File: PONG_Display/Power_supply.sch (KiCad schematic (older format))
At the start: 21 parts, among them J2 Input_Supply+12V, U2 MCP16311MS, U3 LD1117S33TR_SOT223

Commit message: v2
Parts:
- C10, C6, C7: footprint Capacitor_THT:CP_Axial_L10.0mm_D4.5mm_P15.00mm_Horizontal -> Capacitor_THT:CP_Radial_D6.3mm_P2.50mm
- C2, C3: footprint Capacitor_THT:CP_Axial_L10.0mm_D6.0mm_P15.00mm_Horizontal -> Capacitor_THT:CP_Radial_D6.3mm_P2.50mm
- C8: footprint Capacitor_THT:CP_Axial_L10.0mm_D6.0mm_P15.00mm_Horizontal -> Capacitor_SMD:C_Elec_10x10.2
- L1: footprint (none) -> Inductor_SMD:L_12x12mm_H4.5mm
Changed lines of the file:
@@
 F 0 "C8" H 7418 1946 50  0000 L CNN
 F 1 "470u" H 7418 1855 50  0000 L CNN
-F 2 "Capacitor_THT:CP_Axial_L10.0mm_D6.0mm_P15.00mm_Horizontal" H 7338 1750 50  0001 C CNN
+F 2 "Capacitor_SMD:C_Elec_10x10.2" H 7338 1750 50  0001 C CNN
 F 3 "~" H 7300 1900 50  0001 C CNN
 	1    7300 1900
@@
 F 0 "C10" H 8915 1946 50  0000 L CNN
 F 1 "10u" H 8915 1855 50  0000 L CNN
-F 2 "Capacitor_THT:CP_Axial_L10.0mm_D4.5mm_P15.00mm_Horizontal" H 8838 1750 50  0001 C CNN
+F 2 "Capacitor_THT:CP_Radial_D6.3mm_P2.50mm" H 8838 1750 50  0001 C CNN
 F 3 "~" H 8800 1900 50  0001 C CNN
 	1    8800 1900
@@
 F 0 "C3" H 2468 5696 50  0000 L CNN
 F 1 "10u" H 2468 5605 50  0000 L CNN
-F 2 "Capacitor_THT:CP_Axial_L10.0mm_D6.0mm_P15.00mm_Horizontal" H 2388 5500 50  0001 C CNN
+F 2 "Capacitor_THT:CP_Radial_D6.3mm_P2.50mm" H 2388 5500 50  0001 C CNN
 F 3 "~" H 2350 5650 50  0001 C CNN
 	1    2350 5650
@@
 F 0 "C2" H 2118 5696 50  0000 L CNN
 F 1 "10u" H 2118 5605 50  0000 L CNN
-F 2 "Capacitor_THT:CP_Axial_L10.0mm_D6.0mm_P15.00mm_Horizontal" H 2038 5500 50  0001 C CNN
+F 2 "Capacitor_THT:CP_Radial_D6.3mm_P2.50mm" H 2038 5500 50  0001 C CNN
 F 3 "~" H 2000 5650 50  0001 C CNN
 	1    2000 5650
@@
 F 0 "C6" H 5068 5696 50  0000 L CNN
 F 1 "10u" H 5068 5605 50  0000 L CNN
-F 2 "Capacitor_THT:CP_Axial_L10.0mm_D4.5mm_P15.00mm_Horizontal" H 4988 5500 50  0001 C CNN
+F 2 "Capacitor_THT:CP_Radial_D6.3mm_P2.50mm" H 4988 5500 50  0001 C CNN
 F 3 "~" H 4950 5650 50  0001 C CNN
 	1    4950 5650
@@
 F 0 "C7" H 5468 5696 50  0000 L CNN
 F 1 "10u" H 5468 5605 50  0000 L CNN
-F 2 "Capacitor_THT:CP_Axial_L10.0mm_D4.5mm_P15.00mm_Horizontal" H 5388 5500 50  0001 C CNN
+F 2 "Capacitor_THT:CP_Radial_D6.3mm_P2.50mm" H 5388 5500 50  0001 C CNN
 F 3 "~" H 5350 5650 50  0001 C CNN
 	1    5350 5650
@@
 F 0 "L1" V 4840 5500 50  0000 C CNN
 F 1 "22u" V 4749 5500 50  0000 C CNN
-F 2 "" H 4650 5500 50  0001 C CNN
+F 2 "Inductor_SMD:L_12x12mm_H4.5mm" H 4650 5500 50  0001 C CNN
 F 3 "~" H 4650 5500 50  0001 C CNN
 	1    4650 5500

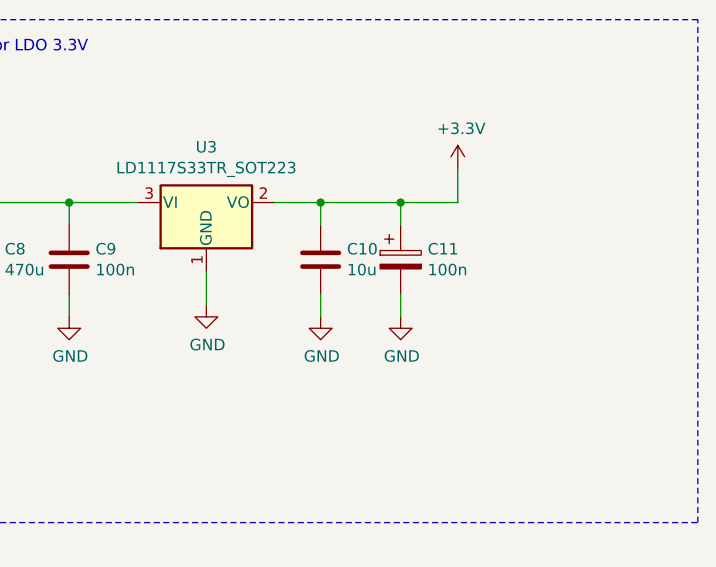
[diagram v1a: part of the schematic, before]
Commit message: Drobne zmiany
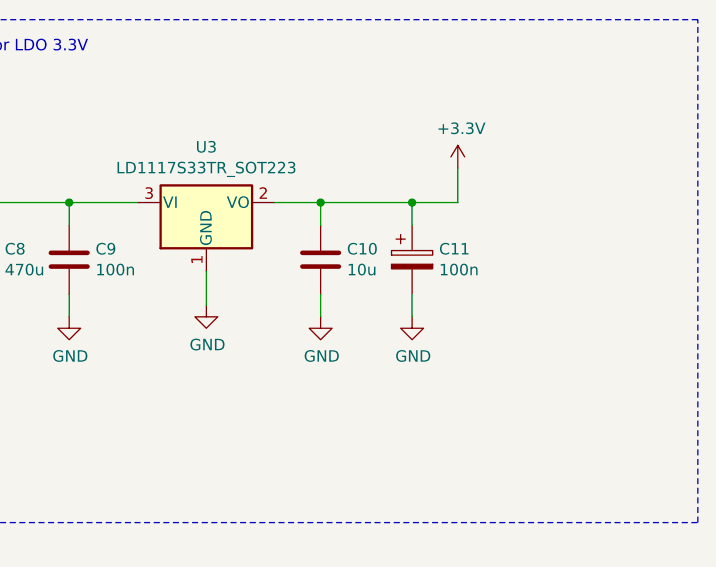
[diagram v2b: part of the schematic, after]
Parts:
- J2: footprint (none) -> TerminalBlock:TerminalBlock_bornier-2_P5.08mm
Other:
- moved on the sheet: C11
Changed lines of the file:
@@
 F 0 "J2" H 1668 1967 50  0000 C CNN
 F 1 "Input_Supply+12V" H 1668 1876 50  0000 C CNN
-F 2 "" H 1750 1750 50  0001 C CNN
+F 2 "TerminalBlock:TerminalBlock_bornier-2_P5.08mm" H 1750 1750 50  0001 C CNN
 F 3 "~" H 1750 1750 50  0001 C CNN
 	1    1750 1750
@@
 L Device:CP C11
 U 1 1 5E8660CC
-P 9150 1900
-F 0 "C11" H 9268 1946 50  0000 L CNN
-F 1 "100n" H 9268 1855 50  0000 L CNN
-F 2 "Capacitor_SMD:C_1206_3216Metric_Pad1.42x1.75mm_HandSolder" H 9188 1750 50  0001 C CNN
-F 3 "~" H 9150 1900 50  0001 C CNN
-	1    9150 1900
+P 9200 1900
+F 0 "C11" H 9318 1946 50  0000 L CNN
+F 1 "100n" H 9318 1855 50  0000 L CNN
+F 2 "Capacitor_SMD:C_1206_3216Metric_Pad1.42x1.75mm_HandSolder" H 9238 1750 50  0001 C CNN
+F 3 "~" H 9200 1900 50  0001 C CNN
+	1    9200 1900
 	1    0    0    -1
 $EndComp
@@
 L power:GND #PWR0114
 U 1 1 5E8670D0
-P 9150 2150
-F 0 "#PWR0114" H 9150 1900 50  0001 C CNN
-F 1 "GND" H 9155 1977 50  0000 C CNN
-F 2 "" H 9150 2150 50  0001 C CNN
-F 3 "" H 9150 2150 50  0001 C CNN
-	1    9150 2150
-	1    0    0    -1
-$EndComp
-Wire Wire Line
-	9150 2050 9150 2150
+P 9200 2150
+F 0 "#PWR0114" H 9200 1900 50  0001 C CNN
+F 1 "GND" H 9205 1977 50  0000 C CNN
+F 2 "" H 9200 2150 50  0001 C CNN
+F 3 "" H 9200 2150 50  0001 C CNN
+	1    9200 2150
+	1    0    0    -1
+$EndComp
+Wire Wire Line
+	9200 2050 9200 2150
 Wire Wire Line
 	8800 2050 8800 2150
@@
 Connection ~ 8800 1650
 Wire Wire Line
-	8800 1650 9150 1650
-Wire Wire Line
-	9150 1650 9150 1750
-Connection ~ 9150 1650
-Wire Wire Line
-	9150 1650 9400 1650
+	8800 1650 9200 1650
+Wire Wire Line
+	9200 1650 9200 1750
+Connection ~ 9200 1650
+Wire Wire Line
+	9200 1650 9400 1650
 $Comp
 L power:+12V #PWR0115
